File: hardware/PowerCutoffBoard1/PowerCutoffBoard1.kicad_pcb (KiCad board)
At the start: 2 copper layers, 50 x 60 mm, 51 parts, among them J1 Conn_Coaxial, J2 Conn_01x03, J3 Conn_01x04, J4 Conn_01x04, J5 Conn_01x04, J6 Conn_01x04, SW1 SW_Push, SW2 SW_Push, SW3 SW_DIP_x04, U1 STM32F303K8Tx, U2 Wio-E5, U3 3.3V, U4 MIC4427, U5 MCP2562-E-SN

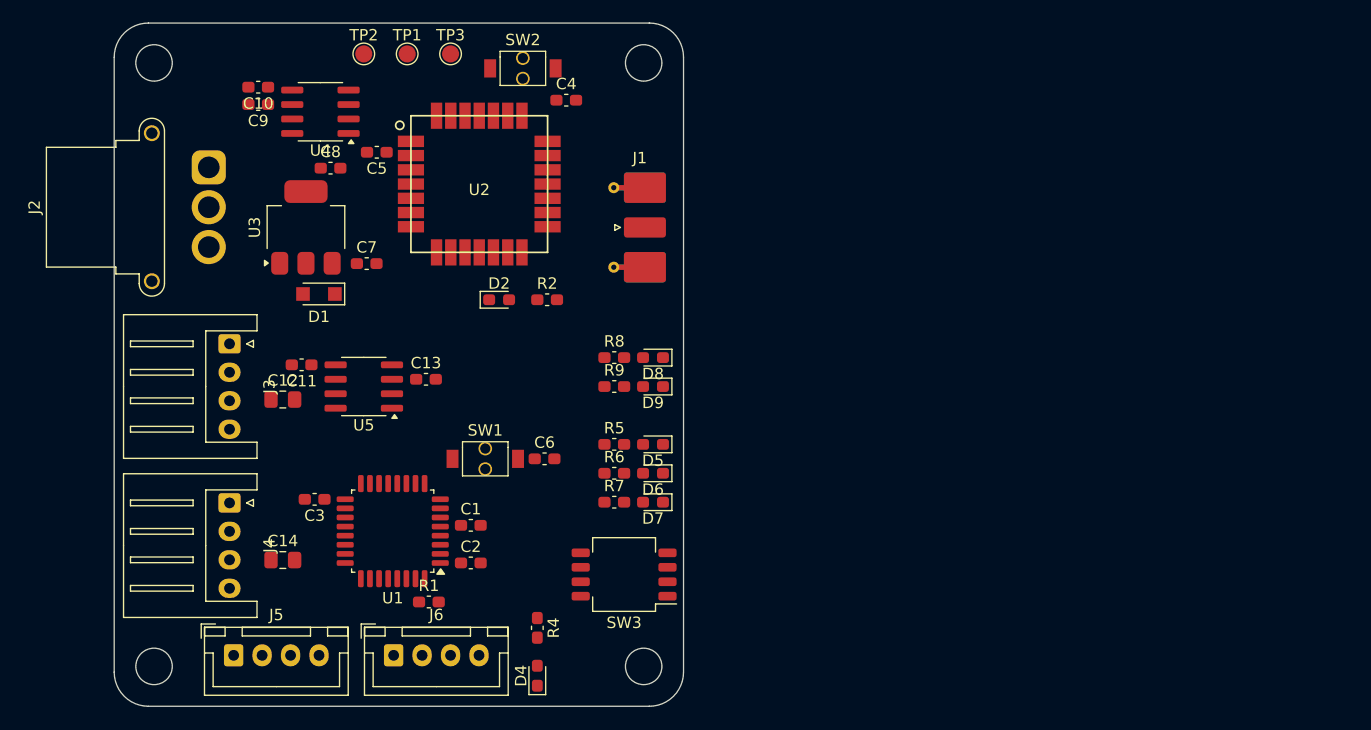
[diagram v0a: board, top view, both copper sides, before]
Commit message: update
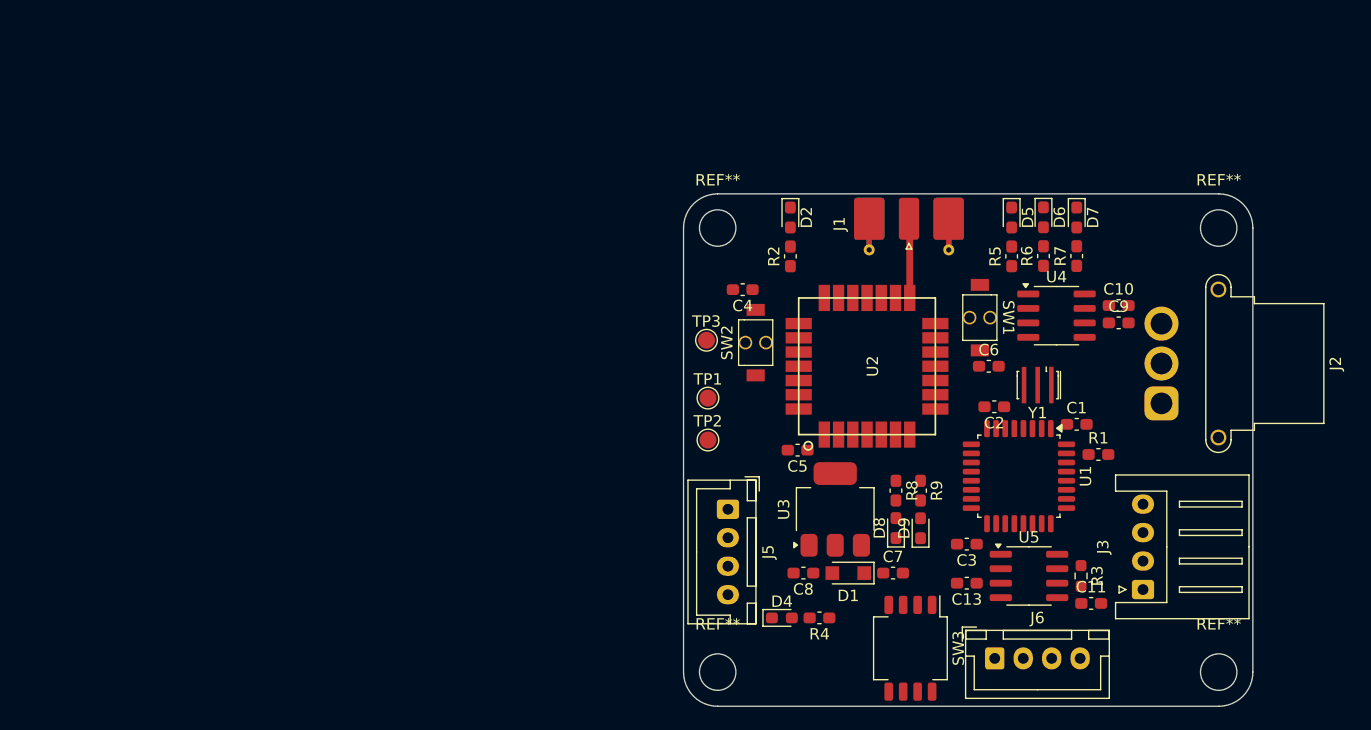
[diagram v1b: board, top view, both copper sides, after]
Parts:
- removed C12, C14: 10u, Capacitor_SMD:C_0805_2012Metric_Pad1.18x1.45mm_HandSolder
- removed J4: Conn_01x04, Connector_JST:JST_XH_S4B-XH-A_1x04_P2.50mm_Horizontal
- removed the REF** at (103.5, 93.5)
- removed the REF** at (146.5, 93.5)
- removed the REF** at (146.5, 146.5)
- removed the REF** at (103.5, 146.5)
- added R3: 120, Resistor_SMD:R_0603_1608Metric_Pad0.98x0.95mm_HandSolder, F.Cu at (184.9, 138.6)
- added REF**: MountingHole_3.2mm_M3, MountingHole:MountingHole_3.2mm_M3, F.Cu at (153.0, 108.0)
- added REF**: MountingHole_3.2mm_M3, MountingHole:MountingHole_3.2mm_M3, F.Cu at (153.0, 147.0)
- added REF**: MountingHole_3.2mm_M3, MountingHole:MountingHole_3.2mm_M3, F.Cu at (197.0, 108.0)
- added REF**: MountingHole_3.2mm_M3, MountingHole:MountingHole_3.2mm_M3, F.Cu at (197.0, 147.0)
- added Y1: Crystal_GND2, Crystal:Resonator_SMD_Murata_CSTxExxV-3Pin_3.0x1.1mm_HandSoldering, F.Cu at (181.1, 121.8)
- moved J2 86.2 mm to (192.0, 123.4), turned to -90 degrees
- moved J3 83.1 mm to (190.4, 139.8), turned to 90 degrees
- moved C10 78.0 mm to (188.2, 114.8), turned to 0 degrees
- moved C9 78.0 mm to (188.2, 116.3), turned to 0 degrees
- moved C11 72.4 mm to (185.8, 141.0), turned to 0 degrees
- moved U4 67.1 mm to (182.8, 115.7), turned to 0 degrees
- moved U5 60.7 mm to (180.3, 138.6), turned to 0 degrees
- moved R1 60.2 mm to (186.4, 127.9)
- moved C3 57.4 mm to (174.9, 135.8)
- moved U1 55.2 mm to (179.5, 129.8), turned to -90 degrees
- moved C8 54.7 mm to (160.5, 138.3), turned to 180 degrees
- moved C1 53.9 mm to (184.5, 125.2)
- moved C7 53.6 mm to (168.4, 138.3)
- moved J6 52.8 mm to (177.3, 145.8)
- moved U3 52.7 mm to (163.3, 132.7)
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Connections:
- J6 pad 1: USART2_RX -> USART1_RX
- J6 pad 3: USART2_TX -> USART1_TX
- U1 pad 2: unconnected-(U1-PF0-Pad2) -> Net-(U1-PF0)
- U1 pad 21: CAN_RX -> CANRX
- U1 pad 22: CAN_TX -> CANTX
- U1 pad 3: unconnected-(U1-PF1-Pad3) -> Net-(U1-PF1)
- U2 pad 10: USART1_RX -> USART2_RX
- U2 pad 9: USART1_TX -> USART2_TX
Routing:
- net Net-(J1-In): track 0.00 -> 6.98 mm
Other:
- board size 50 x 60 mm -> 50 x 45 mm
